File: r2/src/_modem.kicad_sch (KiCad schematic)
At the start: 36 parts, among them J1 , J11 SMA, J12 U_FL-R-SMT-1_10_, J13 JAE_SIM_Card_SF72S006, J2 , J3 , J4 , J5 , J6 , J7 , J8 , J9 , U7 Sierra_Wireless_RC7620, U8 ESD7004, U9 TXS0108EPW

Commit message: Footprint for modem
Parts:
- U7: footprint MODULE_WP7504 -> jeffmakes-footprints:Cellular_Modem-Sierra-Wireless-module-CF3-ringCD

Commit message: Most footprints assigned
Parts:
- C21, C25, C26, C27, C28: footprint (none) -> Capacitor_SMD:C_0603_1608Metric
- C22, C23, C24: footprint (none) -> Capacitor_SMD:C_0805_2012Metric
- J1, J2, J3, J4, J5, J6, J7, J8, J9, TP10, TP11, TP8, TP9: footprint (none) -> TestPoint:TestPoint_Pad_1.0x1.0mm
- J11: footprint (none) -> Connector_Coaxial:SMA_Amphenol_901-144_Vertical
- R21, R22, R23: footprint (none) -> Resistor_SMD:R_0603_1608Metric

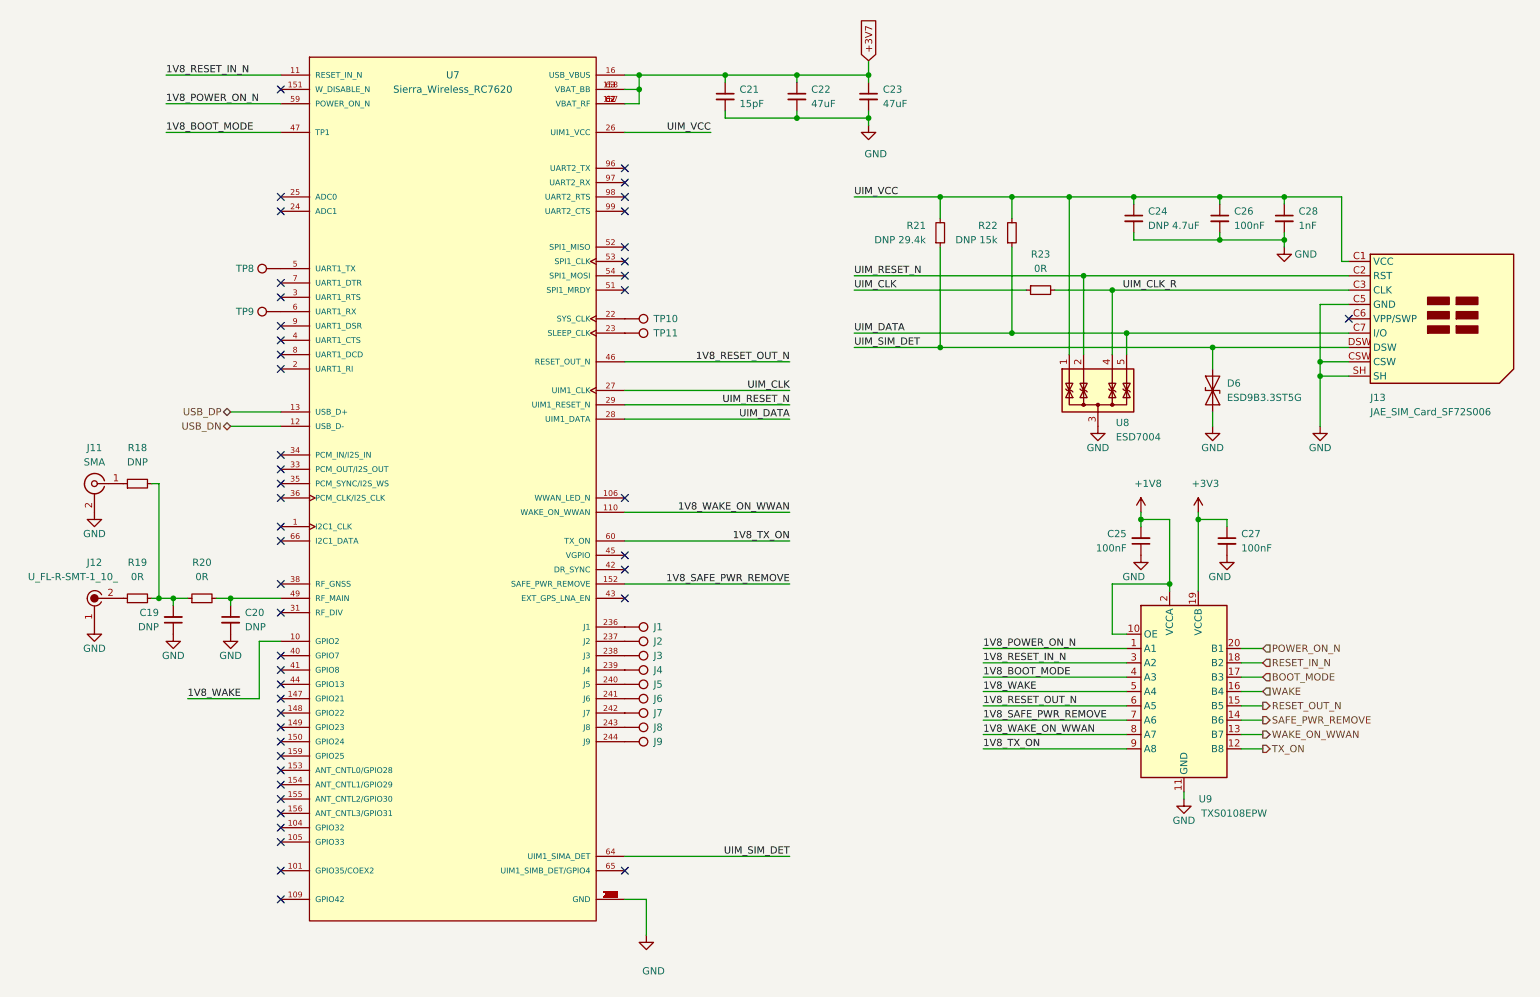
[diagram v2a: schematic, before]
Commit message: All footprints assigned
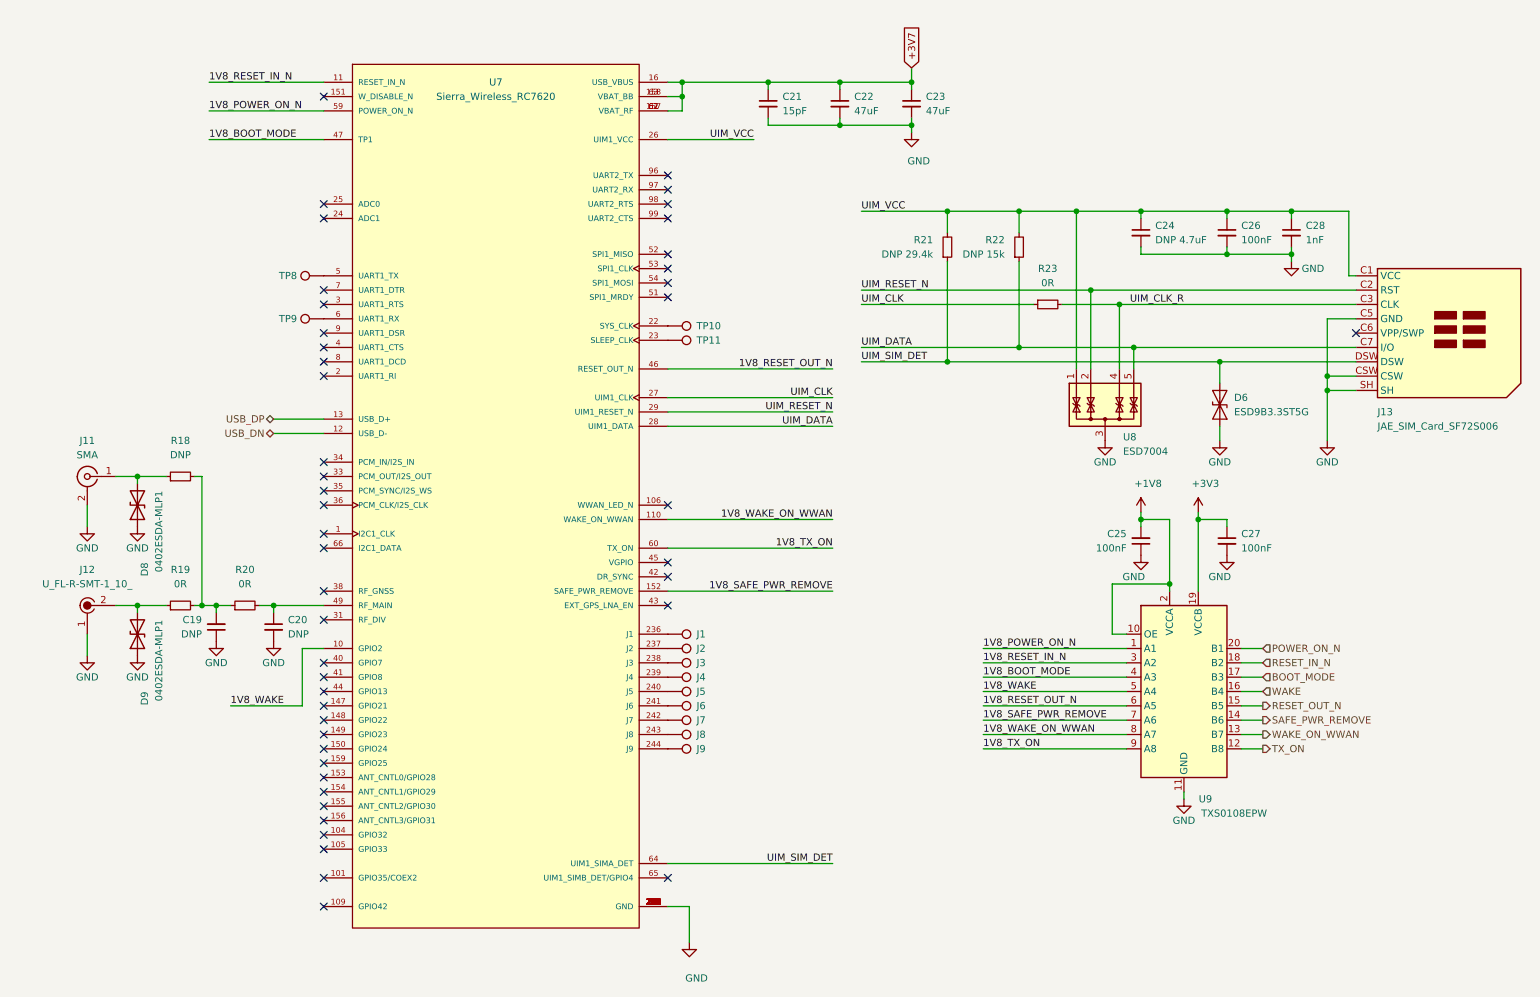
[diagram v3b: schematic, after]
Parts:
- added D8, D9: 0402ESDA-MLP1, Diode_SMD:D_0402_1005Metric, symbol Device:D_TVS
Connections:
- net GND: now also D8.1 (A1), D9.1 (A1)
- net at J11.1 (In), R18.1: now also D8.2 (A2)
- net at J12.2, R19.1: now also D9.2 (A2)
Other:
- moved on the sheet: C19, C20, C21, C22, C23, C24, C26, C28, D6, J1, J11, J12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

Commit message: Change some footprints, change all testpoints to 1mm round.
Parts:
- J1, J2, J3, J4, J5, J6, J7, J8, J9, TP10, TP11, TP8, TP9: footprint TestPoint:TestPoint_Pad_1.0x1.0mm -> TestPoint:TestPoint_Pad_D1.0mm
- U8: footprint Package_SON:USON-10_2.5x1.0mm_P0.5mm -> jeffmakes-footprints:USON-10_2.5x1.0mm_P0.5mm
